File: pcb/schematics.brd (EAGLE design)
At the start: 74.6 x 80 mm, 8 parts, among them IC1 MEGA8-P, X1 22-23-2051, X2 22-23-2051

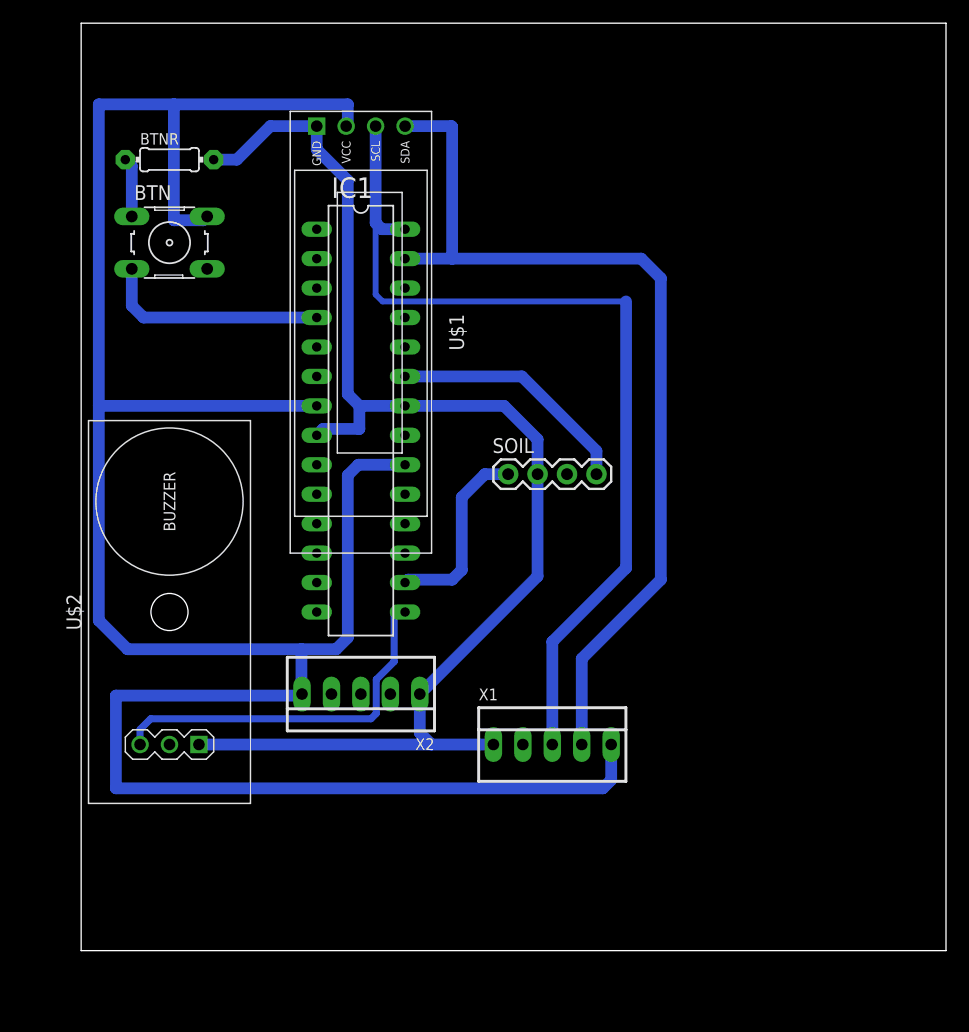
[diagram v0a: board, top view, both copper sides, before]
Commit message: Update eagle files
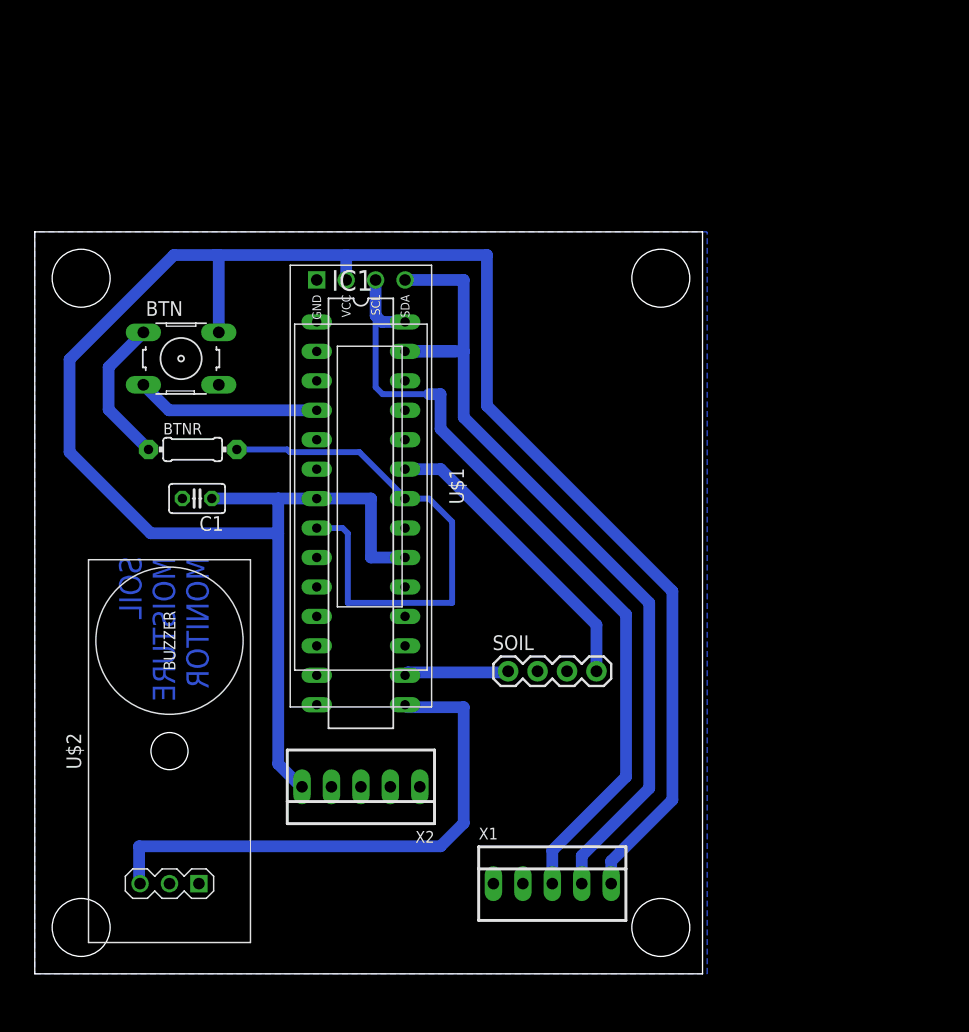
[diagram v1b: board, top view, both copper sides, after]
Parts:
- added C1: (no value), rcl:C025-025X050
- moved BTNR 25.1 mm to (9.62, 43.2)
- moved SOIL 17.0 mm to (36.8, 24.1)
- moved U$1 13.3 mm to (24.1, 40.1)
- moved U$2 12.0 mm to (7.62, 17.2)
- moved X1 12.0 mm to (40.6, 5.78)
- moved BTN 10.0 mm to (8.62, 51.1)
- moved IC1 8.00 mm to (24.1, 37.7)
- moved X2 8.00 mm to (24.1, 14.1)
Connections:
- removed net N$3: BTNR.2, IC1.22, IC1.8, SOIL.2, U$1.1, U$2.1, X1.1, X2.1
- new net GND: BTNR.2, C1.2, IC1.22, IC1.8, SOIL.2, U$1.1, U$2.1, X1.1, X2.1
- net N$5: now also C1.1
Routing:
- net N$3: track 114.6 -> 0.00 mm
- net GND: track 0.00 -> 46.1 mm
- net N$5: track 216.5 -> 188.5 mm
- net N$4: track 32.5 -> 47.2 mm
- net N$2: track 80.0 -> 70.0 mm
- net N$7: track 5.13 -> 12.8 mm
- net N$6: track 16.4 -> 9.03 mm
- net N$1: track 81.3 -> 75.6 mm
- net N$9: track 21.2 -> 26.1 mm
- net N$8: track 19.6 -> 15.9 mm
- added copper zone on layer 16, net GND
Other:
- board size 74.6 x 80 mm -> 57.6 x 64 mm
- board text added: "SOIL MOISTURE MONITOR"

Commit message: Update eagle files
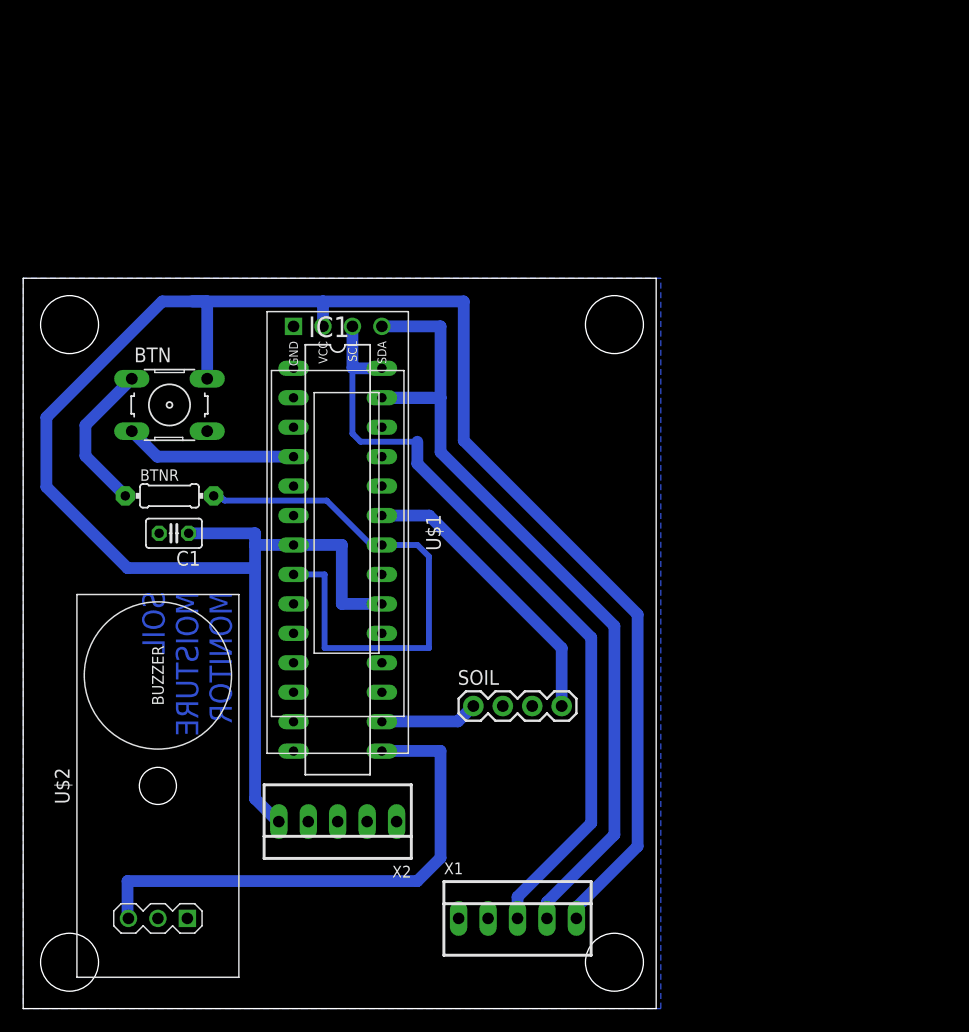
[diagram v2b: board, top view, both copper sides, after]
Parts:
- moved IC1 4.47 mm to (22.1, 33.7)
- moved U$1 4.47 mm to (22.1, 36.1)
- moved BTNR 4.47 mm to (7.62, 39.2)
- moved SOIL 4.24 mm to (33.8, 21.1)
- moved X1 4.24 mm to (37.6, 2.78)
- moved BTN 4.12 mm to (7.62, 47.1)
- moved C1 3.61 mm to (8.00, 36.0)
- moved X2 3.61 mm to (22.1, 11.1)
- moved U$2 3.16 mm to (6.62, 14.2)
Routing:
- net N$2: track 70.0 -> 67.7 mm
- net N$5: track 188.5 -> 186.5 mm
- net N$4: track 47.2 -> 45.4 mm
- net N$1: track 75.6 -> 74.2 mm
- net N$8: track 15.9 -> 14.9 mm
- net N$9: track 26.1 -> 25.2 mm
- net GND: track 46.1 -> 46.7 mm
- net N$6: track 9.03 -> 8.45 mm
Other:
- board size 57.6 x 64 mm -> 54.6 x 63 mm
